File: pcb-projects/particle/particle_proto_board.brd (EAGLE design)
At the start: 33.7 x 27.3 mm, 38 parts, among them IC1 ATTINY20-MMH, IC2 DMC2400V, IC3 DMC2400V, J1 FTS-103-01-L-DV, SW1 T/S-PI SW, SW2 T/S-PI SW, SW3 T/S-PI SW

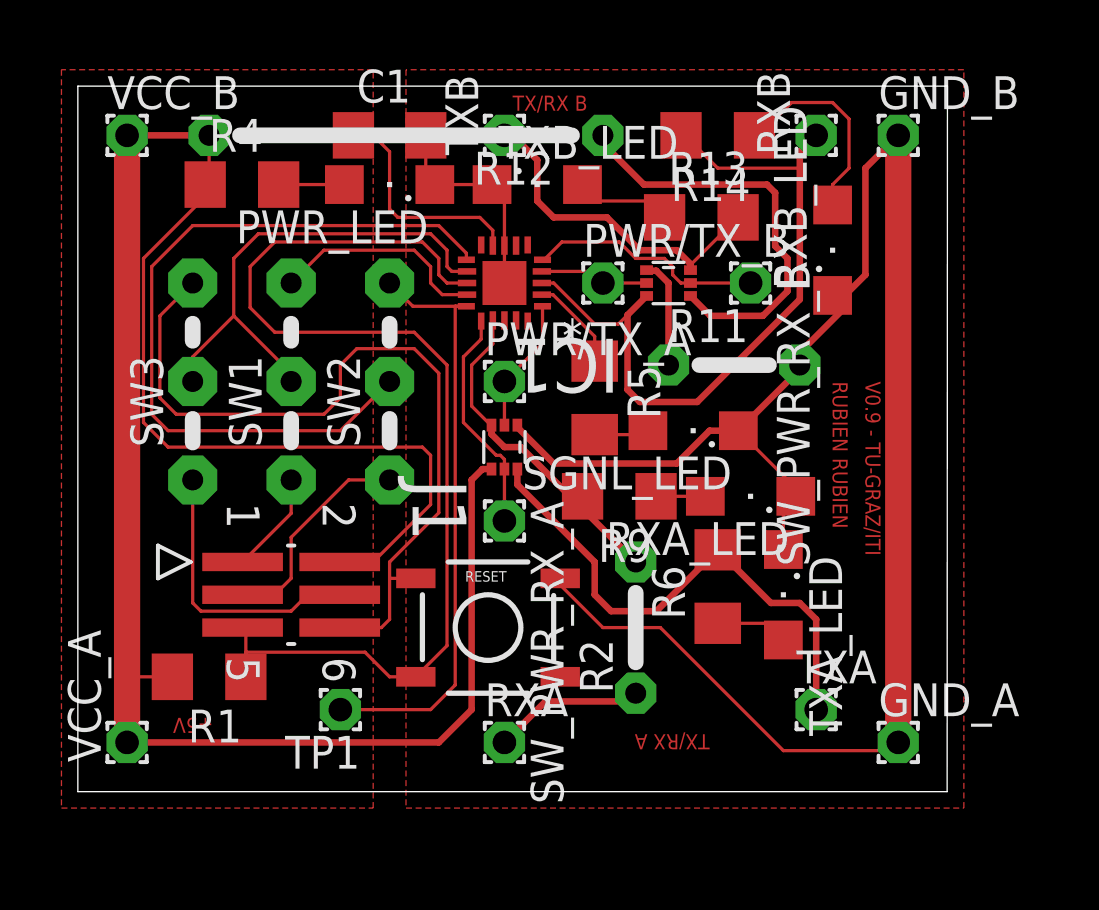
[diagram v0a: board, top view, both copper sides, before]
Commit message: closed #44, closed #43, closed #42
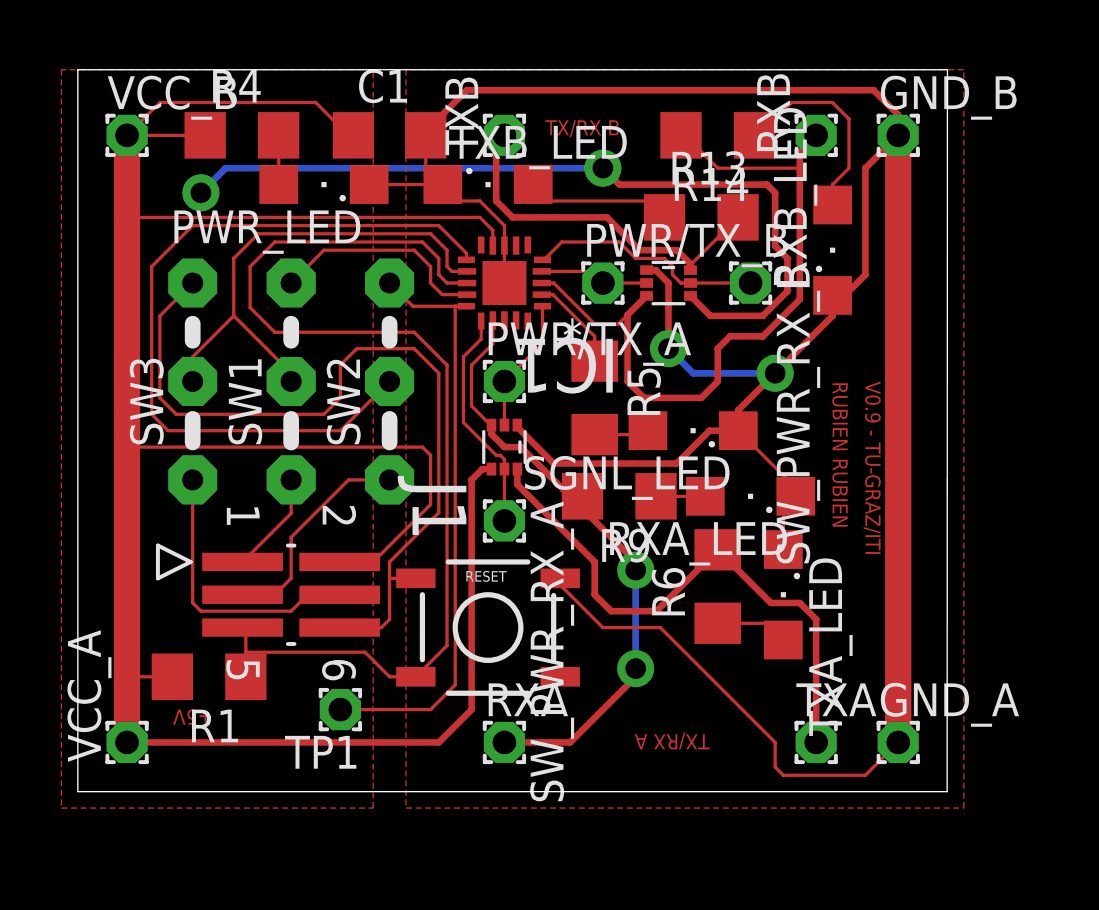
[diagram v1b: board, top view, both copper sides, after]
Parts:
- removed R11: (no value), jumper:05
- removed R12: J15MM, jumper:15
- removed R2: J5MM, jumper:05
- moved PWR_LED 2.54 mm to (10.2, 23.5)
- moved R4 1.90 mm to (6.99, 25.4)
- moved TXB_LED 1.90 mm to (16.5, 23.5)
- moved TXA 1.27 mm to (29.2, 1.91)
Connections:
- removed net N$17: IC3.1, R11.1
- removed net N$2: R2.1, RXA.1
- net GND: now also IC3.1; no longer R11.2
- net RX_A: now also RXA.1; no longer R2.2
- net VCC: no longer R12.1, R12.2
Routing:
- net GND: track 109.7 -> 141.1 mm, vias 0 -> 2
- net VCC: track 107.3 -> 127.0 mm, vias 0 -> 2
- net RX_A: track 13.0 -> 24.0 mm, vias 0 -> 2
- net N$2: track 5.87 -> 0.00 mm
- net N$17: track 4.23 -> 0.00 mm
- net N$13: track 4.34 -> 6.25 mm
- net TX_A: track 20.5 -> 21.8 mm
- net TX_B: track 13.2 -> 14.2 mm
- net N$22: track 2.54 -> 1.91 mm
- net RX_B: track 29.5 -> 28.9 mm
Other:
- board size 33.7 x 27.3 mm -> 33.7 x 27.9 mm
